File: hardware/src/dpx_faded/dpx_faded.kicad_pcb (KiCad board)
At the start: 4 copper layers, 96.5 x 132.7 mm, 62 parts, among them J1 motor.1, J2 motor.2, J3 motor.3, J4 motor.4, SW1 TS-1187A-B-A-B, SW2 TS-1187A-B-A-B, U12 NML0505SC, U5 TC118S, U6 TC118S, U7 TC118S, U8 TC118S, U9 Teensy4.1

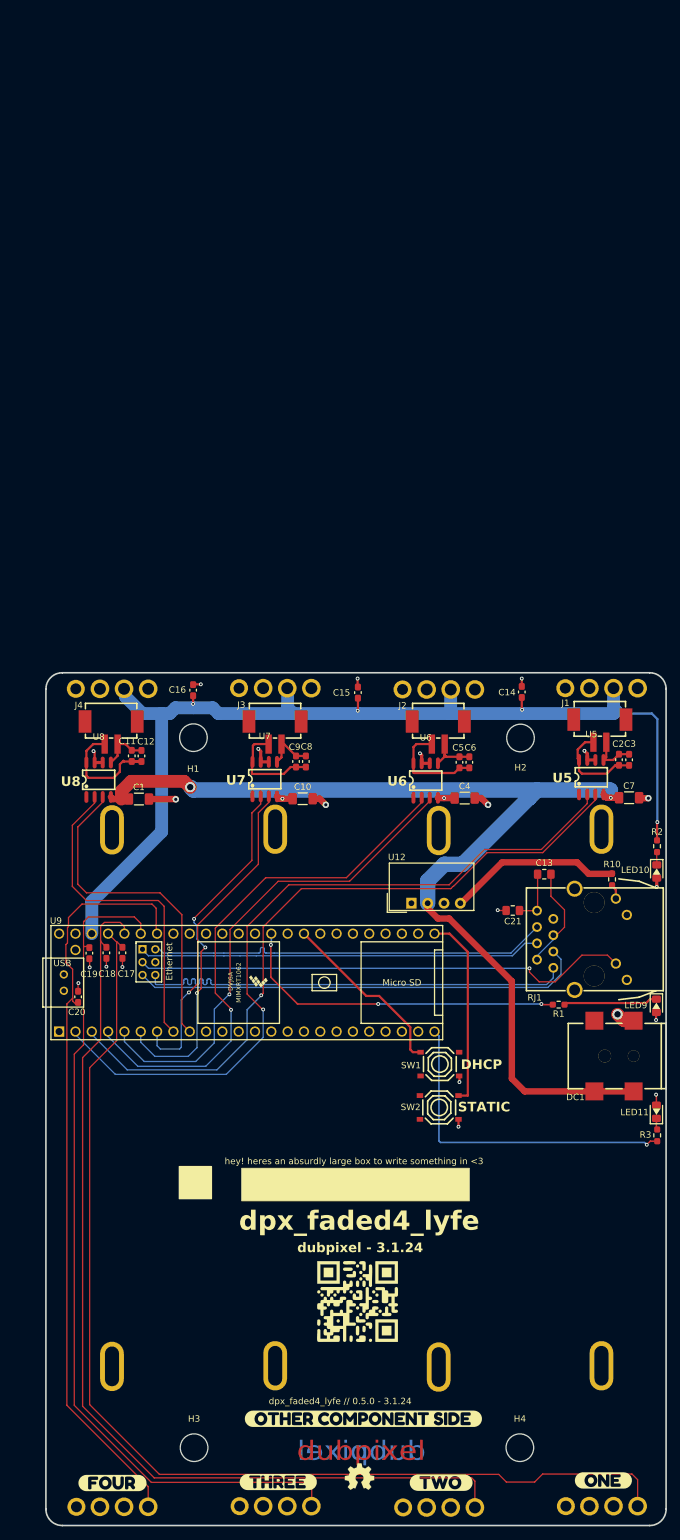
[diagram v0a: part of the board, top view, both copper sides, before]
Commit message: joysticks... but going back to the main branch to make some easier changes
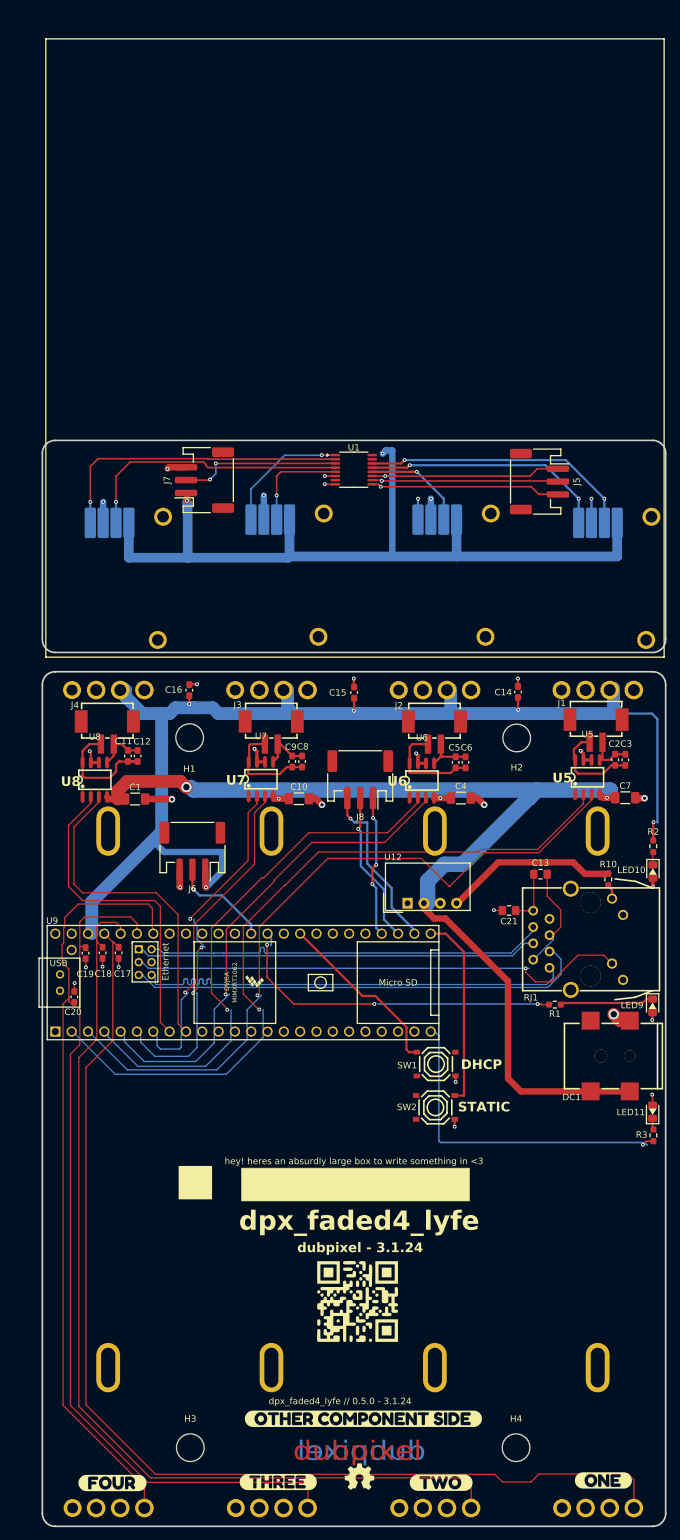
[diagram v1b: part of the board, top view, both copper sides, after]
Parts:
- added J5: Conn_01x03_Socket, Connector_JST:JST_PH_S3B-PH-SM4-TB_1x03-1MP_P2.00mm_Horizontal, F.Cu at (356.4, 76.4)
- added J6: Conn_01x03_Socket, Connector_JST:JST_PH_S3B-PH-SM4-TB_1x03-1MP_P2.00mm_Horizontal, F.Cu at (302.4, 134.0)
- added J7: Conn_01x03_Pin, Connector_JST:JST_PH_S3B-PH-SM4-TB_1x03-1MP_P2.00mm_Horizontal, F.Cu at (304.2, 76.2)
- added J8: Conn_01x03_Pin, Connector_JST:JST_PH_S3B-PH-SM4-TB_1x03-1MP_P2.00mm_Horizontal, F.Cu at (328.5, 122.8)
- added JS1: JOY_PSP, DPX_CONTROL:JOYSTICK-PSP1000_mars, B.Cu at (365.5, 90.8)
- added JS2: JOY_PSP, DPX_CONTROL:JOYSTICK-PSP1000_mars, B.Cu at (340.5, 90.3)
- added JS3: JOY_PSP, DPX_CONTROL:JOYSTICK-PSP1000_mars, B.Cu at (314.5, 90.3)
- added JS4: JOY_PSP, DPX_CONTROL:JOYSTICK-PSP1000_mars, B.Cu at (289.5, 90.8)
- added U1: 74HC4051, Package_SO:TSSOP-16_4.4x5mm_P0.65mm, F.Cu at (327.5, 74.6)
- moved U13 0.66 mm to (314.6, 172.5)
- moved U10 0.66 mm to (365.4, 172.5)
- moved U14 0.62 mm to (289.2, 172.5)
- moved U11 0.60 mm to (340.1, 172.5)
- moved C11 0.59 mm to (292.3, 119.1)
- moved C12 0.59 mm to (293.8, 119.1)
- moved C13 0.59 mm to (356.5, 137.5)
- moved C14 0.59 mm to (353.0, 109.1)
- moved C15 0.59 mm to (327.5, 109.2)
- moved C2 0.59 mm to (368.1, 119.7)
- moved C4 0.59 mm to (344.1, 125.7)
- moved C5 0.59 mm to (343.3, 120.1)
- moved C9 0.59 mm to (317.9, 120.0)
- moved H2 0.59 mm to (352.8, 116.3)
- moved H3 0.59 mm to (302.0, 226.8)
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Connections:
- U9 pad 26: unconnected-(U9-34_RX8-Pad26) -> MUX_1.3
- U9 pad 27: unconnected-(U9-35_TX8-Pad27) -> MUX_1.2
- U9 pad 28: unconnected-(U9-36_CS-Pad28) -> MUX_1.1
- U9 pad 36: unconnected-(U9-14_A0_TX3_SPDIF_OUT-Pad36) -> analog_mux1
- U9 pad 38: unconnected-(U9-16_A2_RX4_SCL1-Pad38) -> wiper_8
- U9 pad 39: unconnected-(U9-17_A3_TX4_SDA1-Pad39) -> wiper_7
- U9 pad 40: unconnected-(U9-18_A4_SDA-Pad40) -> wiper_6
- U9 pad 41: unconnected-(U9-19_A5_SCL-Pad41) -> wiper_5
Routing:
- net +3.3V: track 161.5 -> 308.0 mm, vias 4 -> 6
- net MUX_1.3: track 0.00 -> 56.1 mm, vias 0 -> 2
- net MUX_1.2: track 0.00 -> 52.8 mm, vias 0 -> 2
- net MUX_1.1: track 0.00 -> 51.5 mm, vias 0 -> 4
- net j4.x: track 0.00 -> 47.5 mm, vias 0 -> 1
- net j4.y: track 0.00 -> 42.8 mm, vias 0 -> 1
- net j1.y: track 0.00 -> 42.4 mm, vias 0 -> 2
- net analog_mux1: track 0.00 -> 41.1 mm, vias 0 -> 3
- net j1.x: track 0.00 -> 38.1 mm, vias 0 -> 2
- net GND: track 43.0 -> 66.2 mm, vias 22 -> 31
- net j3.x: track 0.00 -> 20.1 mm, vias 0 -> 1
- net j3.y: track 0.00 -> 16.2 mm, vias 0 -> 1
- net j2.y: track 0.00 -> 16.1 mm, vias 0 -> 1
- net mc3.U: track 56.7 -> 51.5 mm
- net wiper_7: track 0.00 -> 5.17 mm
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- added copper zone on In2.Cu, net GND
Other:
- board size 96.5 x 132.7 mm -> 97 x 169 mm
